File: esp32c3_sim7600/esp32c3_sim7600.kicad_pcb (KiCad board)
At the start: 4 copper layers, 80 parts, among them J1 Conn_01x04_Socket, J2 Conn_01x04_Socket, J3 2171790001, J4 CONUFL001-SMD-T, J5 CONUFL001-SMD-T, J6 CONUFL001-SMD-T, J7 SIM7050-6-0-00-X_REVC, Q1 NPN, Q2 NPN, Q3 NPN, SW1 SW_Push, SW2 SW_Push, U1 ESP32-C3-MINI-1-N4, U2 AMS1117-3.3, U3 USBLC6-2P6, U4 SIM7600E, U5 MIC29302AWD, U6 TXB0108RGY

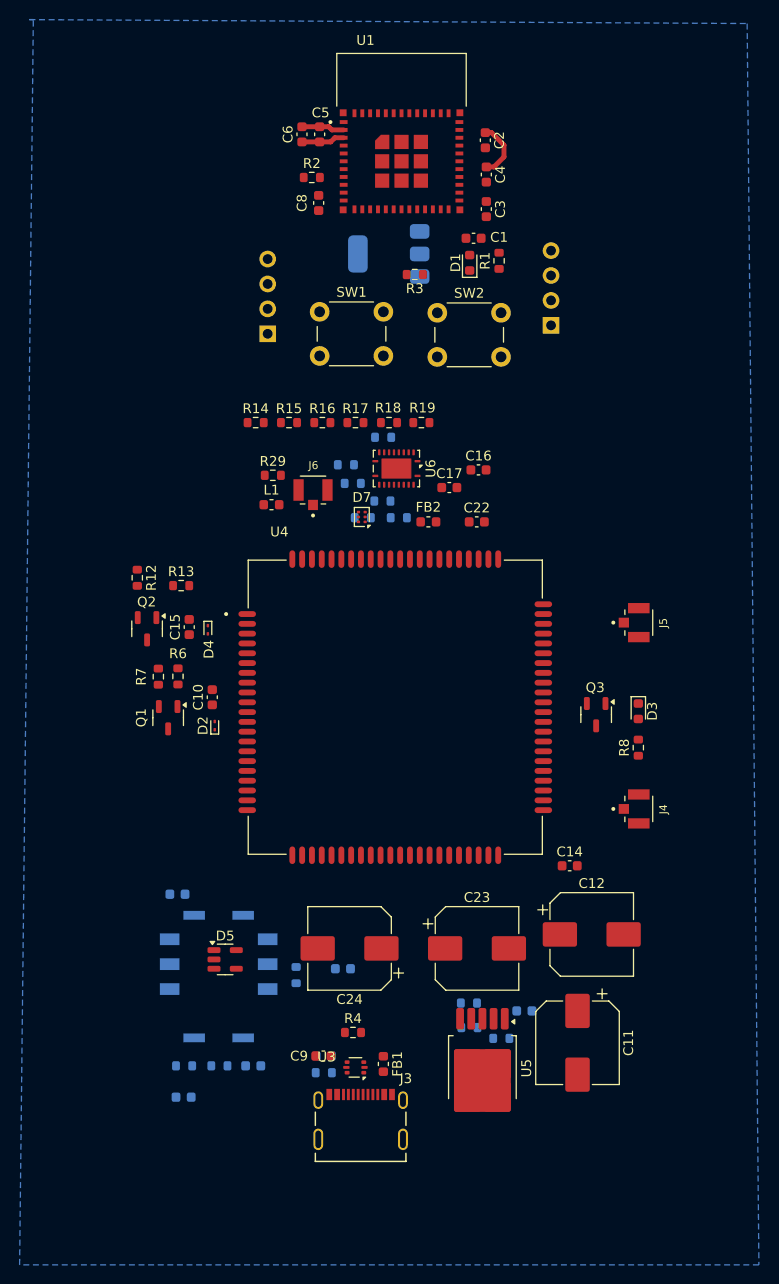
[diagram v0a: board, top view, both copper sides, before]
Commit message: completed routing
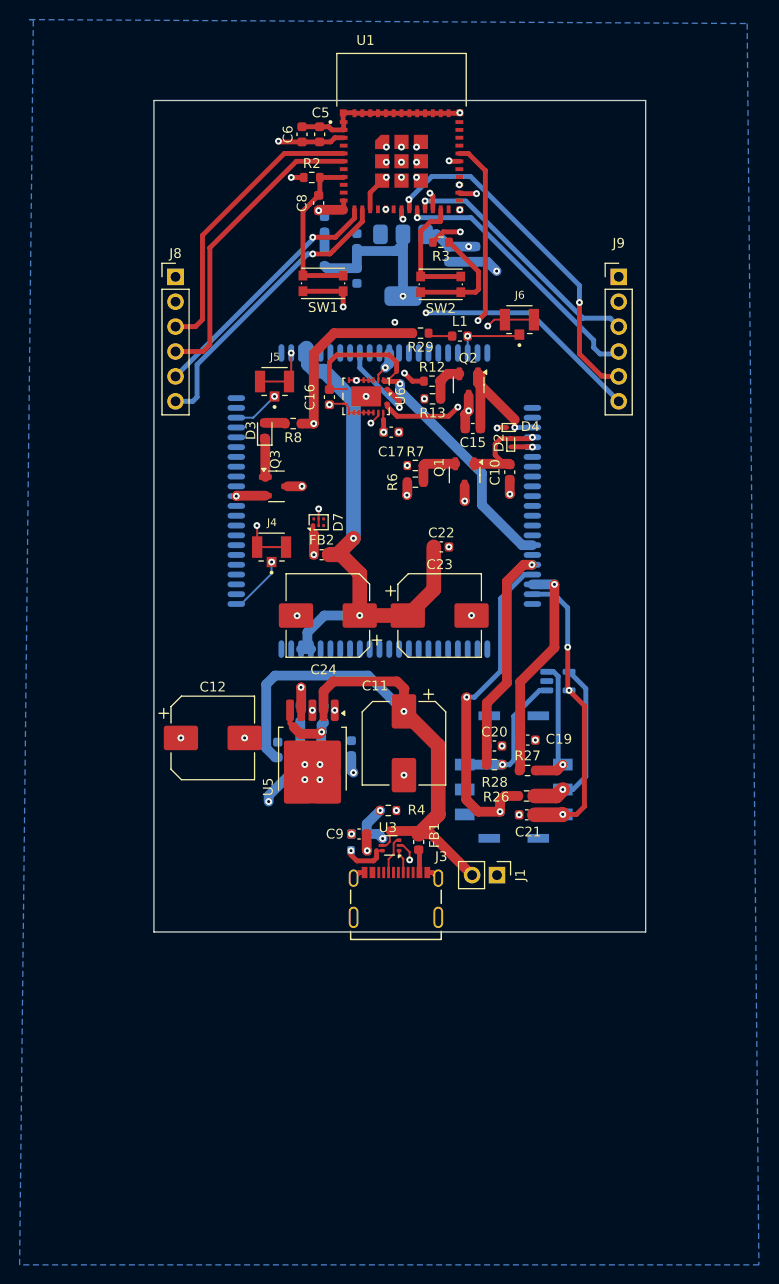
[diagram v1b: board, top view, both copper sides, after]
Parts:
- removed J2: Conn_01x04_Socket, Connector_PinHeader_2.54mm:PinHeader_1x04_P2.54mm_Vertical
- removed R14, R15, R16, R17, R18, R19, R20, R21, R22, R23, R24, R25: 47K, Resistor_SMD:R_0603_1608Metric
- added J8: Conn_01x06_Pin, Connector_PinHeader_2.54mm:PinHeader_1x06_P2.54mm_Vertical, F.Cu at (163.3, 49.6)
- added J9: Conn_01x06_Pin, Connector_PinHeader_2.54mm:PinHeader_1x06_P2.54mm_Vertical, F.Cu at (208.5, 49.6)
- C1, C14, C2, C3, C4, D1, D5, R1, U4: moved to B.Cu
- C19, C20, C21, R26, R27, R28: moved to F.Cu
- J1: value Conn_01x04_Socket -> Conn_01x02_Pin; footprint Connector_PinHeader_2.54mm:PinHeader_1x04_P2.54mm_Vertical -> Connector_PinHeader_2.54mm:PinHeader_1x02_P2.54mm_Vertical; moved to F.Cu
- SW1, SW2: footprint Button_Switch_THT:SW_PUSH_6mm -> Button_Switch_SMD:SW_Push_1P1T_NO_CK_KMR2
- moved J1 60.0 mm to (196.1, 110.7), turned to -90 degrees
- moved R8 48.3 mm to (175.3, 64.6), turned to 180 degrees
- moved D3 47.7 mm to (172.4, 65.3), turned to 90 degrees
- moved J4 46.0 mm to (173.1, 77.2), turned to 0 degrees
- moved J5 44.6 mm to (173.4, 60.3), turned to 0 degrees
- moved R26 44.5 mm to (199.1, 102.6), turned to 0 degrees
- moved D5 44.2 mm to (202.3, 90.9)
- moved C12 43.5 mm to (167.1, 96.7)
- moved R27 43.5 mm to (199.2, 100.0), turned to 0 degrees
- moved C19 43.4 mm to (199.2, 96.9)
- moved C18 42.9 mm to (195.6, 104.2)
- moved D2 41.8 mm to (197.5, 66.6)
- moved Q2 41.2 mm to (193.2, 60.7)
- moved Q3 40.1 mm to (173.6, 71.0), turned to 0 degrees
- moved Q1 39.1 mm to (192.8, 69.8)
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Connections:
- J1 pad 1: /esp32c3/IO0 -> GND
- J1 pad 2: /esp32c3/IO1 -> /power/5V_VBUS
- U6 pad 12: Net-(U6-B8) -> GND
- U6 pad 13: Net-(U6-B7) -> GND
- U6 pad 14: Net-(U6-B6) -> GND
- U6 pad 15: Net-(U6-B5) -> GND
- U6 pad 16: Net-(U6-B4) -> GND
- U6 pad 17: Net-(U6-B3) -> GND
- U6 pad 4: Net-(U6-A3) -> GND
- U6 pad 5: Net-(U6-A4) -> GND
- U6 pad 6: Net-(U6-A5) -> GND
- U6 pad 7: Net-(U6-A6) -> GND
- U6 pad 8: Net-(U6-A7) -> GND
- U6 pad 9: Net-(U6-A8) -> GND
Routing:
- net /power/5V_VBUS: track 5.85 -> 120.1 mm, vias 0 -> 2
- net GND: track 4.38 -> 81.9 mm, vias 0 -> 47
- net D+: track 0.00 -> 74.1 mm, vias 0 -> 2
- net D-: track 0.00 -> 68.1 mm, vias 0 -> 2
- net /sim7600/VBAT: track 0.00 -> 55.1 mm, vias 0 -> 2
- net 3V3: track 4.43 -> 43.5 mm, vias 0 -> 4
- net /sim7600/VDD_1V8: track 0.00 -> 39.0 mm, vias 0 -> 1
- net ESP_SIM_RESET: track 0.00 -> 38.8 mm, vias 0 -> 2
- net ESP_TX0: track 0.00 -> 36.9 mm, vias 0 -> 2
- net SIM_VBAT: track 0.00 -> 36.9 mm, vias 0 -> 6
- net /esp32c3/IO5: track 0.00 -> 35.9 mm, vias 0 -> 2
- net /esp32c3/IO4: track 0.00 -> 35.0 mm, vias 0 -> 2
- net /sim7600/USIM_RST: track 0.00 -> 33.8 mm, vias 0 -> 2
- net ESP_RX0: track 0.00 -> 32.6 mm, vias 0 -> 2
- net /esp32c3/IO3: track 0.00 -> 31.0 mm
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- added copper zone on In2.Cu, net 3V3
- added copper zone on In1.Cu, net GND
- removed copper zone on In1.Cu, net 3V3
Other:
- board outline added: 50.2 x 84.8 mm
